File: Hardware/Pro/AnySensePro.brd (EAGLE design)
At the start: 30 x 45 mm, 63 parts, among them U1 LP2992IM5-3.3, U2 BLUENRGQTR, U3 SN65HVD232D, U4 STM32F303RET6, U5 BALF-NRG-01D3, U6 M25P16VMN6P, X6 MEM2051-00-195-00-A, X7 TC2030-IDC-NL, Y1 ABM3B, Y2 ABM8, Y3 ABS07

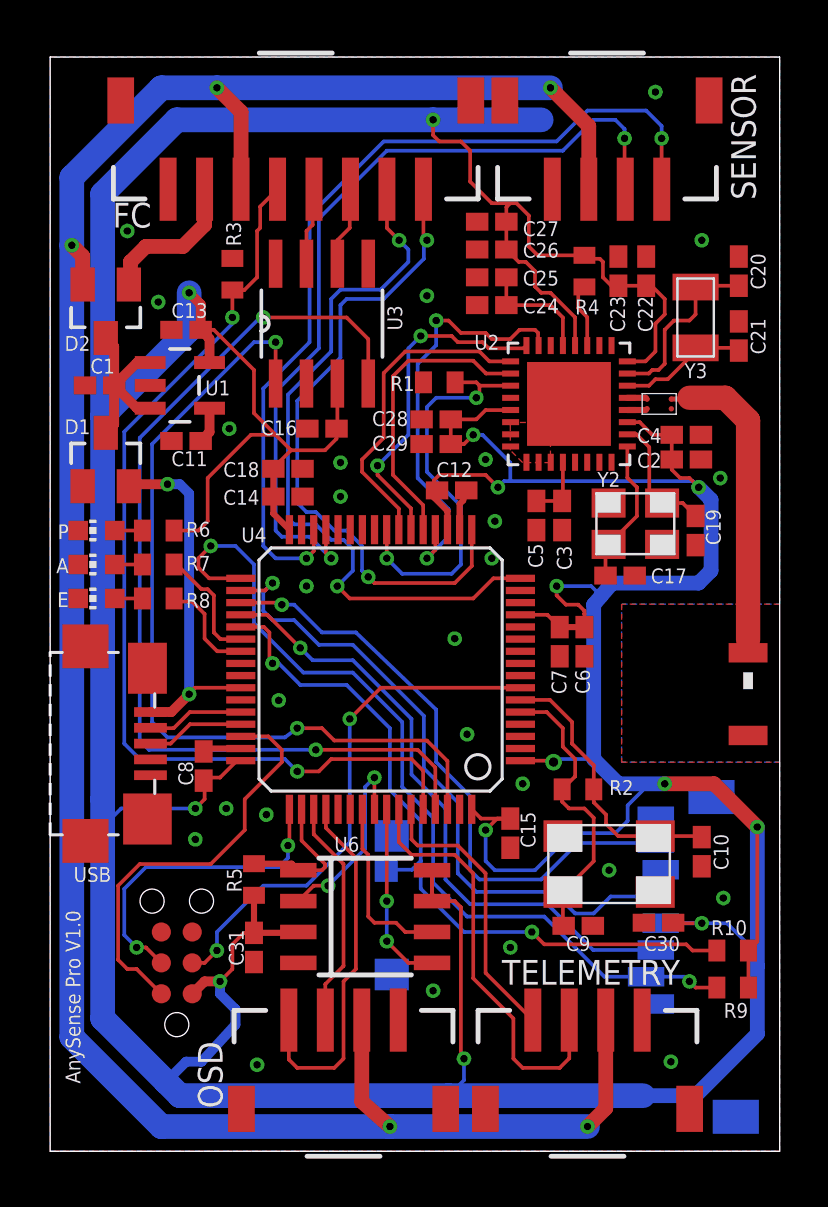
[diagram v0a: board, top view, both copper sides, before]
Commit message: Hardware redesign
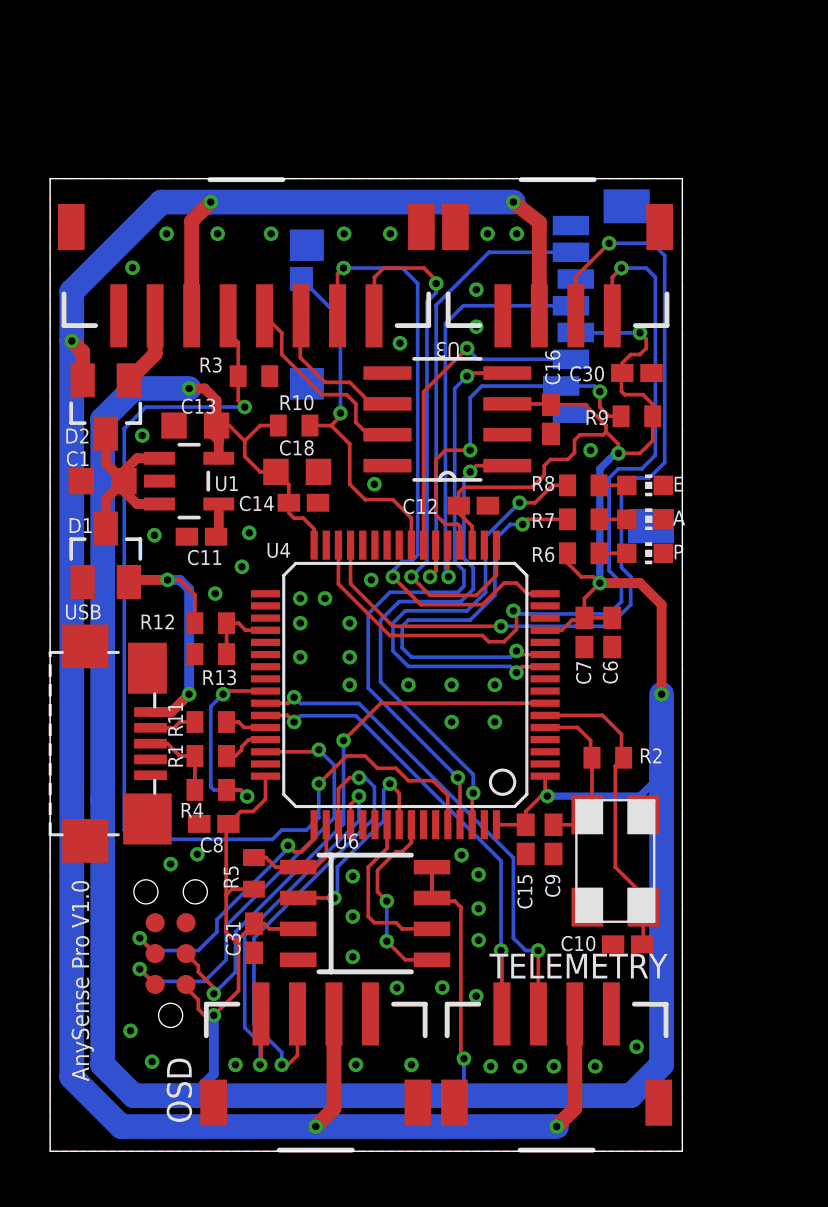
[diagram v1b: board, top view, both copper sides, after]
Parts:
- removed A1: 2450AT18A100, johanson-technology:2450AT18A100E
- removed C17, C19: 15pF, rcl:C0402K
- removed C2, C22, C26, C28: 1uF, rcl:C0402K
- removed C20, C21: 22pF, rcl:C0402K
- removed C23, C27, C29, C4, C5: 100nF, rcl:C0402K
- removed C24, C3: 100pF, rcl:C0402K
- removed C25: 150nF, rcl:C0402K
- removed U2: BLUENRGQTR, ST-Microelctronics:QFN32
- removed U5: BALF-NRG-01D3, ST-Microelctronics:BALF-NRG-01D3
- removed Y2: ABM8, abracon:3.2X2.5MM
- removed Y3: ABS07, abracon:ABS07
- added R11: 22R, rcl:R0402
- added R12: 10K, rcl:R0402
- added R13: 15K, rcl:R0402
- C1, C13, C18: device rcl:C0402K -> rcl:C0603K
- R1: value 10K -> 22R
- R4: value 10K -> 1.5K
- moved R10 28.1 mm to (10.0, 29.8), turned to 180 degrees
- moved R4 26.3 mm to (6.60, 14.9), turned to 0 degrees
- moved X6 24.5 mm to (17.8, 32.4)
- moved R9 23.8 mm to (24.1, 30.2)
- moved E 23.0 mm to (24.5, 27.4), turned to 270 degrees
- moved A 22.6 mm to (24.5, 26.0), turned to 270 degrees
- moved C30 22.6 mm to (24.1, 32.0), turned to 0 degrees
- moved P 22.6 mm to (24.5, 24.6), turned to 270 degrees
- moved R8 18.1 mm to (21.9, 27.4), turned to 180 degrees
- moved R1 18.0 mm to (6.60, 16.3), turned to 180 degrees
- moved R7 17.6 mm to (21.9, 26.0), turned to 180 degrees
- moved R6 17.5 mm to (21.9, 24.6), turned to 180 degrees
- moved C16 9.43 mm to (20.6, 30.1), turned to 270 degrees
- moved U3 6.49 mm to (16.3, 30.1), turned to 180 degrees
- moved FC 5.59 mm to (8.07, 37.0)
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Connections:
- removed net BLE_IRQ: R1.2, U2.3, U4.24
- removed net N$10: C19.1, U2.18, Y2.3
- removed net N$11: C17.2, U2.17, Y2.1
- removed net N$12: C3.1, C5.1, U2.12
- removed net N$13: C20.1, U2.23, Y3.2
- removed net N$14: C21.1, U2.22, Y3.1
- removed net N$2: U2.21, U5.1
- removed net N$3: U2.20, U5.2
- removed net N$4: C24.1, C25.1, U2.29
- removed net N$5: R4.2, U2.27
- removed net N$9: A1.1, U5.4
- removed net SPI2_MISO: U4.35, X6.7
- removed net SPI2_MOSI: U4.36, X6.3
- removed net SPI2_NSS: R9.1, U4.33, X6.2
- removed net SPI2_SCK: U4.34, X6.5
- new net USB_D+: R1.2, R4.1, USB.3
- new net USB_D-: R11.2, USB.2
- new net USB_DISCONNECT: R4.2, U4.41
- new net USB_SENSE: R12.1, R13.2, U4.36
- net +3V3: no longer C2.1, C22.1, C23.1, C26.1, C27.1, C28.1, C29.1, C4.1, R4.1, U2.19, U2.24, U2.28, U2.5
- net +5V/2: now also R12.2; no longer U4.42
- net GND: now also R13.1; no longer C17.1, C19.2, C2.2, C20.2, C21.2, C22.2, C23.2, C24.2, C25.2, C26.2, C27.2, C28.2, C29.2, C3.2, C4.2, C5.2, R1.1, U2.10, U2.11, U2.30, U2.6, U2.7, U2.8, U2.9, U2.P$1, U5.3, Y2.2, Y2.4
- net LED_ACTIVITY: now also U4.11; no longer U4.38
- net LED_ERROR: now also U4.10; no longer U4.39
- net SD_CD: now also U4.24; no longer U4.37
- net SPI1_MISO: now also X6.7; no longer U2.32
- net SPI1_MOSI: now also X6.3; no longer U2.1
- net SPI1_NSS: now also R9.1, X6.2; no longer U2.31
- net SPI1_SCK: now also X6.5; no longer U2.2
- net USART1_RX: now also U4.43; no longer U4.59
- net USART1_TX: now also U4.42; no longer U4.58
- net USB_DM: now also R11.1; no longer USB.2
- net USB_DP: now also R1.1; no longer USB.3
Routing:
- net +3V3: track 269.2 -> 171.2 mm, vias 14 -> 8
- net SPI2_NSS: track 35.9 -> 0.00 mm, vias 2 -> 0
- net SPI2_SCK: track 27.3 -> 0.00 mm, vias 1 -> 0
- net SPI2_MOSI: track 25.8 -> 0.00 mm, vias 1 -> 0
- net SPI2_MISO: track 25.4 -> 0.00 mm, vias 1 -> 0
- net BLE_IRQ: track 16.8 -> 0.00 mm, vias 2 -> 0
- net SD_CD: track 30.5 -> 14.7 mm, vias 2 -> 1
- net CANRX: track 40.4 -> 25.4 mm
- net LED_ERROR: track 4.24 -> 18.7 mm, vias 0 -> 2
- net CANTX: track 35.0 -> 21.1 mm
- net N$9: track 13.1 -> 0.00 mm
- net LED_ACTIVITY: track 4.91 -> 17.0 mm, vias 0 -> 2
- net UART4_TX: track 9.49 -> 19.8 mm, vias 0 -> 2
- net USB_DISCONNECT: track 0.00 -> 8.47 mm, vias 0 -> 2
- net N$13: track 7.56 -> 0.00 mm
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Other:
- board size 30 x 45 mm -> 26 x 40 mm
